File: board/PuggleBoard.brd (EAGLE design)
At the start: 54.6 x 86.4 mm, 133 parts, among them U1 LMP7704, U10 SN65LVDS2, U11 SN65LVDS1, U12 SN65LVDS1, U13 SN65LVDS1, U14 SN65MLVD201D, U15 24C, U2 ADS8331, U3 OPA4209, U4 AD5686, U5 LTM8045, U6 TPS7A3001, U7 TPS7A4901, U8 REF5040, U9 AD8032

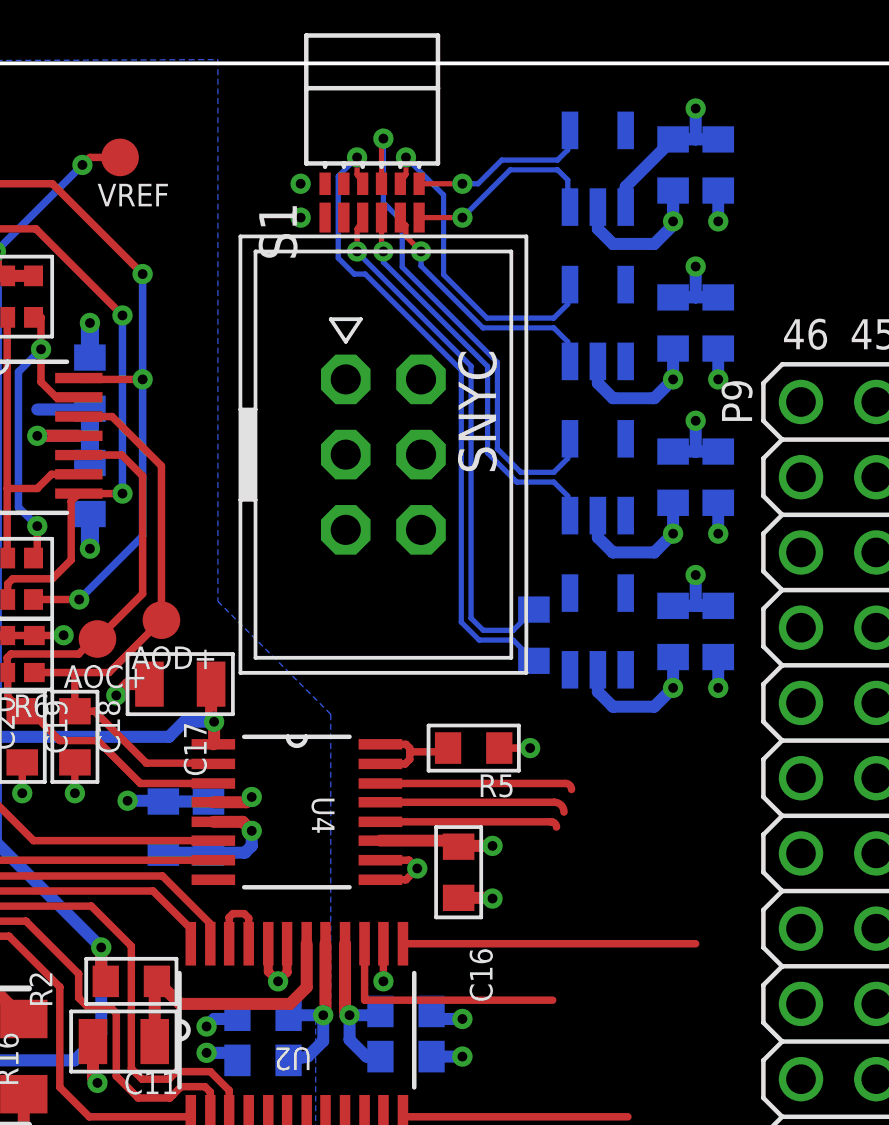
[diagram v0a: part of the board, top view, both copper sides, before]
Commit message: A few minor changes.
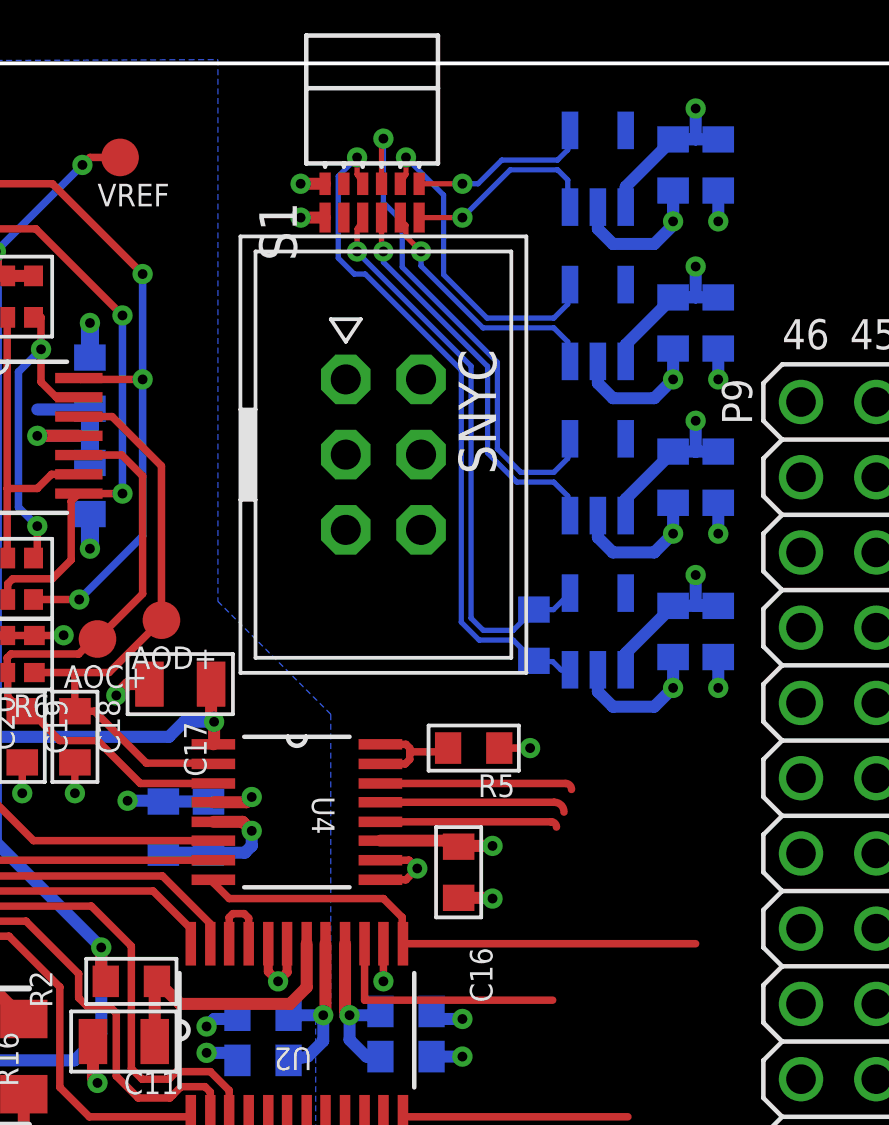
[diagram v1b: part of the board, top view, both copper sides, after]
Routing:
- net VDRIVE: track 36.6 -> 45.9 mm
- net SPI4: track 9.88 -> 17.7 mm
- net MISO1_N: track 17.8 -> 19.3 mm
- net MISO1_P: track 21.8 -> 23.2 mm
- net GND: track 115.6 -> 116.4 mm
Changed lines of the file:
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@@
 <layers>
 <layer number="1" name="Top" color="12" fill="1" visible="yes" active="yes"/>
-<layer number="2" name="GND" color="12" fill="3" visible="no" active="yes"/>
+<layer number="2" name="GND" color="12" fill="3" visible="yes" active="yes"/>
 <layer number="3" name="Route3" color="4" fill="3" visible="no" active="no"/>
 <layer number="4" name="Route4" color="1" fill="4" visible="no" active="no"/>
@@
 <layer number="13" name="Route13" color="4" fill="5" visible="no" active="no"/>
 <layer number="14" name="Route14" color="1" fill="6" visible="no" active="no"/>
-<layer number="15" name="PWR" color="1" fill="6" visible="no" active="yes"/>
+<layer number="15" name="PWR" color="1" fill="6" visible="yes" active="yes"/>
 <layer number="16" name="Bottom" color="1" fill="1" visible="yes" active="yes"/>
 <layer number="17" name="Pads" color="10" fill="1" visible="yes" active="yes"/>
@@
 <wire x1="46.609" y1="69.088" x2="46.609" y2="68.06155" width="0.4064" layer="16"/>
 <wire x1="46.609" y1="68.06155" x2="46.86269375" y2="68.06155" width="0.4064" layer="16"/>
+<wire x1="45.847" y1="78.4606" x2="44.2468" y2="76.8604" width="0.4064" layer="16"/>
+<wire x1="44.2468" y1="76.8604" x2="44.2468" y2="76.3016" width="0.4064" layer="16"/>
+<wire x1="45.847" y1="73.2536" x2="44.2468" y2="71.6534" width="0.4064" layer="16"/>
+<wire x1="44.2468" y1="71.6534" x2="44.2468" y2="71.0946" width="0.4064" layer="16"/>
+<wire x1="45.847" y1="68.0466" x2="44.2468" y2="66.4464" width="0.4064" layer="16"/>
+<wire x1="44.2468" y1="66.4464" x2="44.2468" y2="65.8876" width="0.4064" layer="16"/>
+<wire x1="33.274" y1="82.296" x2="34.0995" y2="82.296" width="0.4064" layer="1"/>
 <wire x1="66.3194" y1="55.626" x2="66.3194" y2="57.658" width="0" layer="19" extent="1-1"/>
 <wire x1="68.8848" y1="52.705" x2="66.3194" y2="55.626" width="0" layer="19" extent="1-1"/>
 <wire x1="47.371" y1="68.0466" x2="66.3194" y2="57.658" width="0" layer="19" extent="1-16"/>
 <wire x1="11.5316" y1="8.001" x2="11.684" y2="8.001" width="0" layer="19" extent="1-1"/>
-<wire x1="34.0995" y1="82.296" x2="33.274" y2="82.296" width="0" layer="19" extent="1-1"/>
 <wire x1="37.3126" y1="47.371" x2="38.354" y2="47.371" width="0" layer="19" extent="1-1"/>
-<wire x1="44.2468" y1="76.3016" x2="45.847" y2="78.4606" width="0" layer="19" extent="16-16"/>
-<wire x1="44.2468" y1="71.0946" x2="45.847" y2="73.2536" width="0" layer="19" extent="16-16"/>
-<wire x1="44.2468" y1="65.8876" x2="45.847" y2="68.0466" width="0" layer="19" extent="16-16"/>
 </signal>
 <signal name="VDD_5V">
@@
 <wire x1="42.545" y1="41.785" x2="42.547" y2="41.783" width="1.016" layer="1"/>
 <wire x1="42.547" y1="41.783" x2="44.45" y2="41.783" width="1.016" layer="1"/>
+<wire x1="33.274" y1="81.153" x2="34.0995" y2="81.153" width="0.4064" layer="1"/>
 <wire x1="68.0466" y1="55.626" x2="68.0466" y2="57.658" width="0" layer="19" extent="1-1"/>
 <wire x1="68.8848" y1="48.895" x2="68.0466" y2="55.626" width="0" layer="19" extent="1-1"/>
@@
 <wire x1="26.162" y1="76.4286" x2="26.162" y2="76.327" width="0" layer="19" extent="16-16"/>
 <wire x1="31.1404" y1="52.705" x2="31.242" y2="52.832" width="0" layer="19" extent="16-16"/>
-<wire x1="34.0995" y1="81.153" x2="33.274" y2="81.153" width="0" layer="19" extent="1-1"/>
 </signal>
 <signal name="BAT_SENSE">
@@
 <contactref element="BB1" pad="76"/>
 <wire x1="36.7284" y1="56.642" x2="46.609" y2="56.642" width="0.254" layer="1"/>
+<wire x1="30.3276" y1="58.801" x2="30.3276" y2="58.6994" width="0.254" layer="1"/>
+<wire x1="30.3276" y1="58.6994" x2="30.861" y2="58.166" width="0.254" layer="1"/>
+<wire x1="30.861" y1="58.166" x2="36.068" y2="58.166" width="0.254" layer="1"/>
+<wire x1="36.068" y1="58.166" x2="36.703" y2="57.531" width="0.254" layer="1"/>
+<wire x1="36.703" y1="57.531" x2="36.703" y2="56.6674" width="0.254" layer="1"/>
+<wire x1="36.703" y1="56.6674" x2="36.7284" y2="56.642" width="0.254" layer="1"/>
 <wire x1="46.609" y1="56.642" x2="50.165" y2="54.61" width="0" layer="19" extent="1-1"/>
-<wire x1="30.3276" y1="58.801" x2="36.7284" y2="56.642" width="0" layer="19" extent="1-1"/>
 </signal>
 <signal name="BOARD_TEMP">
@@
 <wire x1="39.3016125" y1="66.8909" x2="40.4495" y2="66.8909" width="0.1778" layer="16"/>
 <wire x1="40.4495" y1="66.8909" x2="41.148" y2="66.1924" width="0.1778" layer="16"/>
-<wire x1="41.148" y1="66.1924" x2="42.3672" y2="65.8876" width="0" layer="19" extent="16-16"/>
+<wire x1="41.148" y1="66.1924" x2="41.1734" y2="66.167" width="0.1778" layer="16"/>
+<wire x1="41.1734" y1="66.167" x2="41.783" y2="66.167" width="0.1778" layer="16"/>
+<wire x1="41.783" y1="66.167" x2="42.0624" y2="65.8876" width="0.1778" layer="16"/>
+<wire x1="42.0624" y1="65.8876" x2="42.3672" y2="65.8876" width="0.1778" layer="16"/>
 </signal>
 <signal name="MISO1_N" class="2">
@@
 <wire x1="39.4383875" y1="67.2211" x2="40.4495" y2="67.2211" width="0.1778" layer="16"/>
 <wire x1="40.4495" y1="67.2211" x2="41.148" y2="67.9196" width="0.1778" layer="16"/>
-<wire x1="41.148" y1="67.9196" x2="42.3672" y2="68.4784" width="0" layer="19" extent="16-16"/>
+<wire x1="41.148" y1="67.9196" x2="41.8084" y2="67.9196" width="0.1778" layer="16"/>
+<wire x1="41.8084" y1="67.9196" x2="42.3672" y2="68.4784" width="0.1778" layer="16"/>
 </signal>
 <signal name="N$8">
